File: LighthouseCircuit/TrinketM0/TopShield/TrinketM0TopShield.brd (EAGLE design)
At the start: 15.2 x 15.2 mm, 23 parts

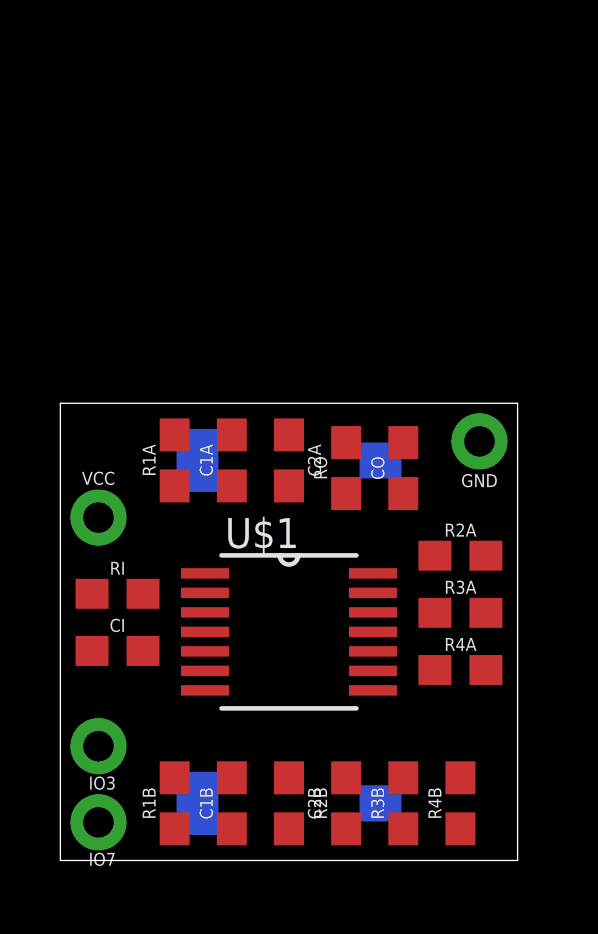
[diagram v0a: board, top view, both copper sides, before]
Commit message: Zippies can now perform perfectly synchronous drive along any predefined path.
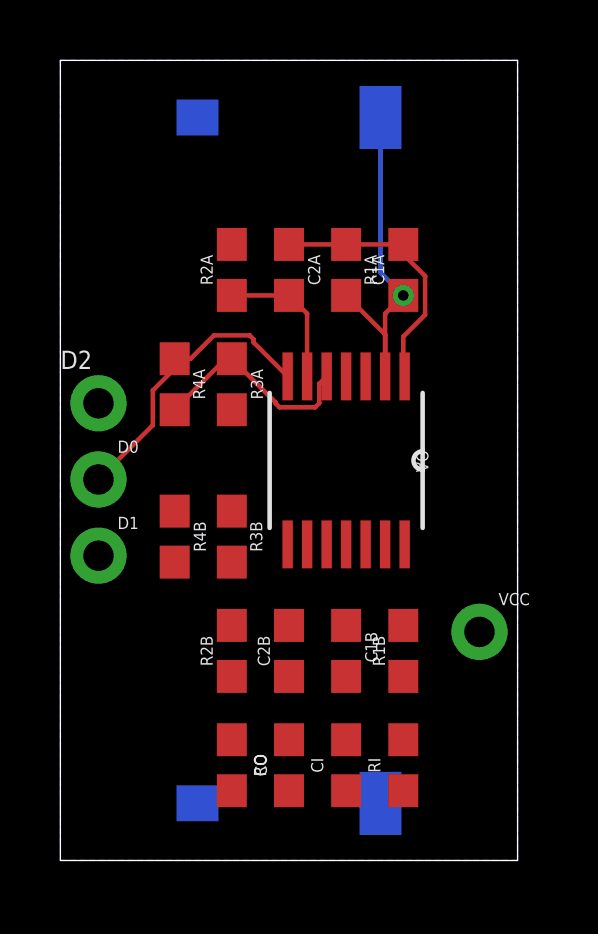
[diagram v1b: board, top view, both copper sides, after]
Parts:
- removed GND: SINGLE-THROUGH-HOLE, ZippyComponentLibrary:SINGLE-THROUGH-HOLE
- removed IO3, IO7: (no value), SparkFun-Connectors:1X01_NO_SILK
- removed U$1: TLV2464IPW, ZippyComponentLibrary:PW14
- added D0: (no value), SparkFun-Connectors:1X01_NO_SILK
- added DI0, DI1: PHOTODIODEBPW, ZippyComponentLibrary:BPW34_BP104_SMD
- added OA: TLV2464IPW, ZippyComponentLibrary:PW14
- D1, D2: value PHOTODIODEBPW -> (none); device ZippyComponentLibrary:BPW34_BP104_SMD -> SparkFun-Connectors:1X01_NO_SILK
- moved R4A 13.5 mm to (3.81, 15.9), turned to 90 degrees
- moved VCC 13.3 mm to (14.0, 7.62)
- moved R4B 13.0 mm to (3.81, 10.8), turned to 270 degrees
- moved R2A 12.2 mm to (5.71, 19.7), turned to 90 degrees
- moved CO 11.4 mm to (5.71, 3.17), turned to 270 degrees
- moved RI 11.1 mm to (11.4, 3.17), turned to 90 degrees
- moved R3A 10.8 mm to (5.71, 15.9), turned to 270 degrees
- moved R3B 10.6 mm to (5.71, 10.8), turned to 90 degrees
- moved D1 10.4 mm to (1.27, 10.2), flipped to the top
- moved RO 10.1 mm to (7.62, 3.17), turned to 90 degrees
- moved R1B 9.16 mm to (11.4, 6.99)
- moved C1A 8.54 mm to (11.4, 19.7)
- moved R1A 8.54 mm to (9.53, 19.7)
- moved CI 8.52 mm to (9.53, 3.17), turned to 90 degrees
- moved D2 6.63 mm to (1.27, 15.2), flipped to the top
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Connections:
- removed net IO3: IO3.1, R4A.2, U$1.8
- removed net IO7: IO7.1, R4B.2, U$1.14
- new net D0: D0.1, OA.7, R4A.2
- new net D1: D1.1, OA.8, R4B.2
- net D1IN: now also DI1.CATHODE, OA.13; no longer D2.CATHODE, U$1.2
- net D1OA2P: now also OA.9; no longer U$1.13
- net D1OAOUT1: now also OA.14; no longer U$1.1
- net D2IN: now also DI0.CATHODE, OA.2; no longer D1.CATHODE, U$1.6
- net D2OA1OUT: now also OA.1; no longer U$1.7
- net D2OA2N: now also OA.5; no longer U$1.10
- net D2OA2P: now also OA.6; no longer U$1.9
- net GND: now also D2.1, OA.11; no longer GND.1, U$1.11
- net LVCC: now also DI0.ANODE, DI1.ANODE, OA.12, OA.3; no longer D1.ANODE, D2.ANODE, U$1.3, U$1.5
- net N$11: now also OA.10; no longer U$1.12
- net VCC: now also OA.4; no longer U$1.4
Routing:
- net D2IN: track 0.00 -> 12.4 mm, vias 0 -> 1
- net D0: track 0.00 -> 9.79 mm
- net D2OA1OUT: track 0.00 -> 8.83 mm
- net D2OA2N: track 0.00 -> 7.26 mm
- net D2OA2P: track 0.00 -> 4.86 mm
- added copper zone on layer 16, net GND
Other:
- board size 15.2 x 15.2 mm -> 15.2 x 26.7 mm
- board text removed: "Designed, Manufactured, and Assembled by Kyle Davis"
